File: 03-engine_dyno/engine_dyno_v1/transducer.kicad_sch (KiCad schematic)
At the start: 15 parts, among them J2 Screw_Terminal_01x05, U6 INA827AIDGKR, U7 AD630ARZ, U8 OPA192IDBVR, U9 ADS1120IPWR

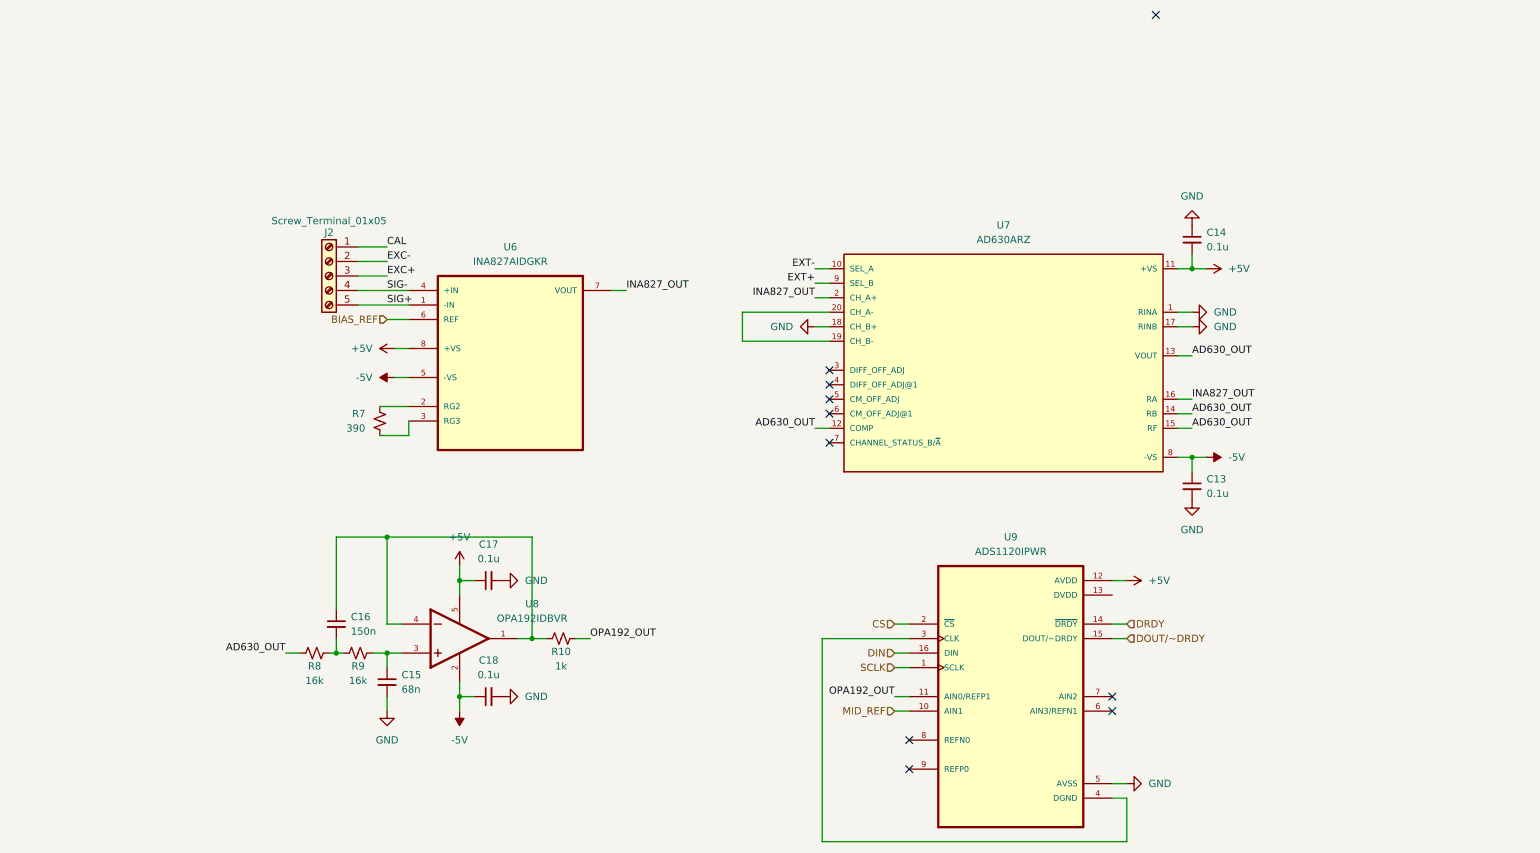
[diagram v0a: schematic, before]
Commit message: clean up
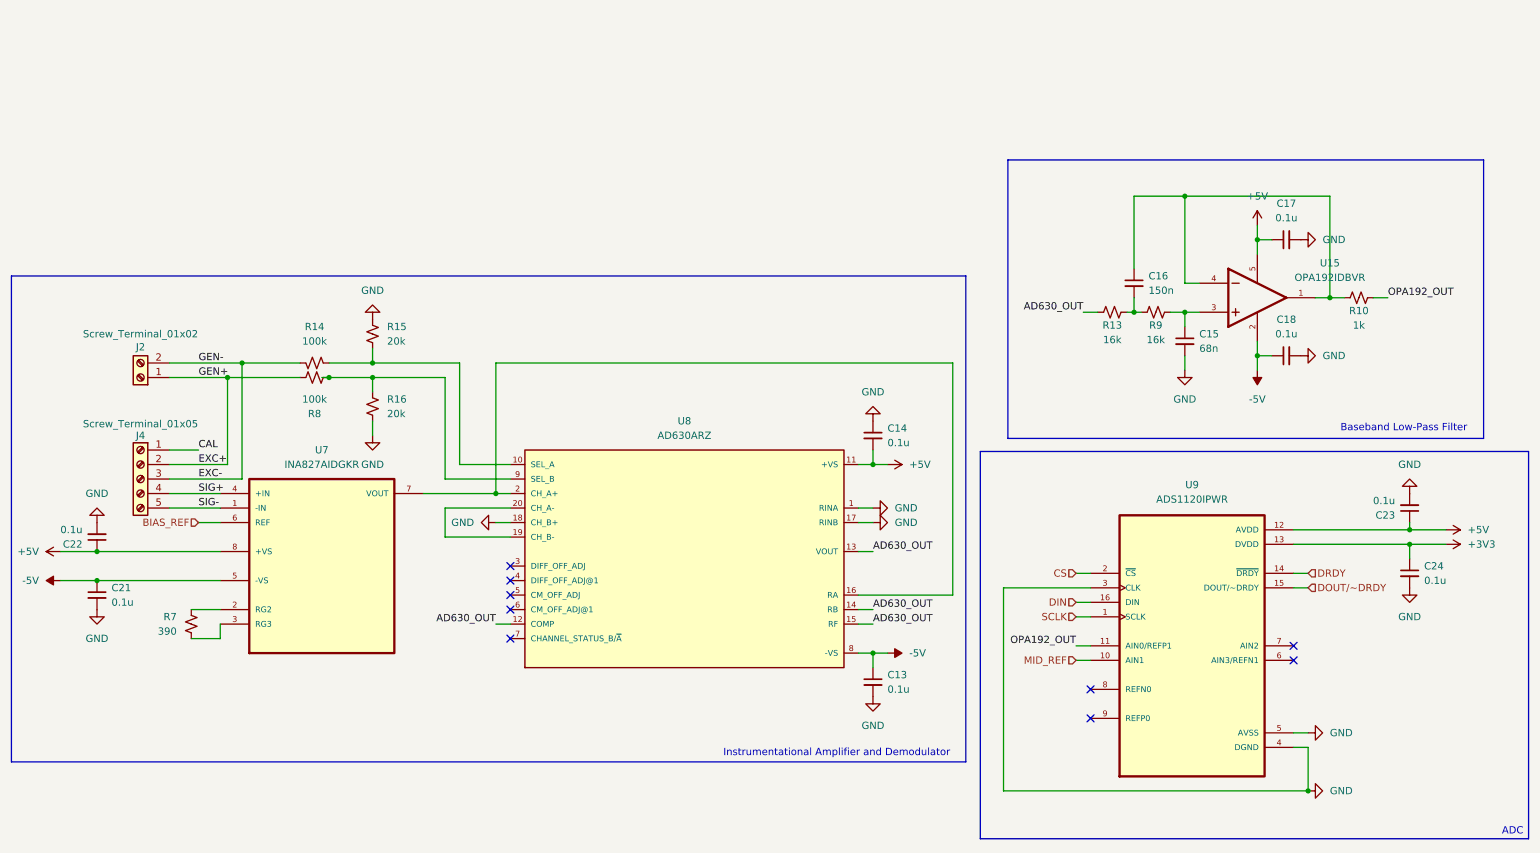
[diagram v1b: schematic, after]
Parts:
- added C21, C22, C23, C24: 0.1u, symbol Device:C_Small
- added J2: Screw_Terminal_01x02, symbol Connector:Screw_Terminal_01x02
- added R14, R8: 100k, symbol Device:R_Small_US
- added R15, R16: 20k, symbol Device:R_Small_US
- renumbered J2 to J4, R8 to R13, U8 to U15, U6 to U7, U7 to U8
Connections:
- net +5V: now also C22.1, C23.1
- net -5V: now also C21.1
- net EXC+: now also J4.2 (Pin_2), J2.1 (Pin_1), R8.1; no longer J4.3 (Pin_3)
- net EXC-: now also J4.3 (Pin_3), J2.2 (Pin_2), R14.1; no longer J4.2 (Pin_2)
- net GND: now also U9.3 (CLK), U9.4 (DGND), C21.2, C22.2, C23.2, C24.2, R15.2, R16.1
- net SIG+: now also J4.4 (Pin_4), U7.4 (+IN); no longer J4.5 (Pin_5), U7.1 (-IN)
- net SIG-: now also J4.5 (Pin_5), U7.1 (-IN); no longer J4.4 (Pin_4), U7.4 (+IN)
- net +3V3: now reaches U9.13 (DVDD)
- net +3V3: now also C24.1
- net EXT+: no longer names the net of U8.9 (SEL_B)
- net EXT+: now also R16.2, R8.2
- net EXT-: no longer names the net of U8.10 (SEL_A)
- net EXT-: now also R14.2, R15.1
- net INA827_OUT: no longer names the net of U7.7 (VOUT), U8.16 (RA), U8.2 (CH_A+)
- no-connect marks 10 -> 9
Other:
- note added: "ADC"
- note added: "Baseband Low-Pass Filter"
- note added: "Instrumentational Amplifier and Demodulator"
- moved on the sheet: C13, C14, C15, C16, C17, C18, J4, R10, R13, R7, R9, U15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
